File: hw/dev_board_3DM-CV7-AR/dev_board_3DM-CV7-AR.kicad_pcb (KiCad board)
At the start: 4 copper layers, 26 parts, among them J1 87438-0643, U1 DMP2240UW, U2 DMP2240UW

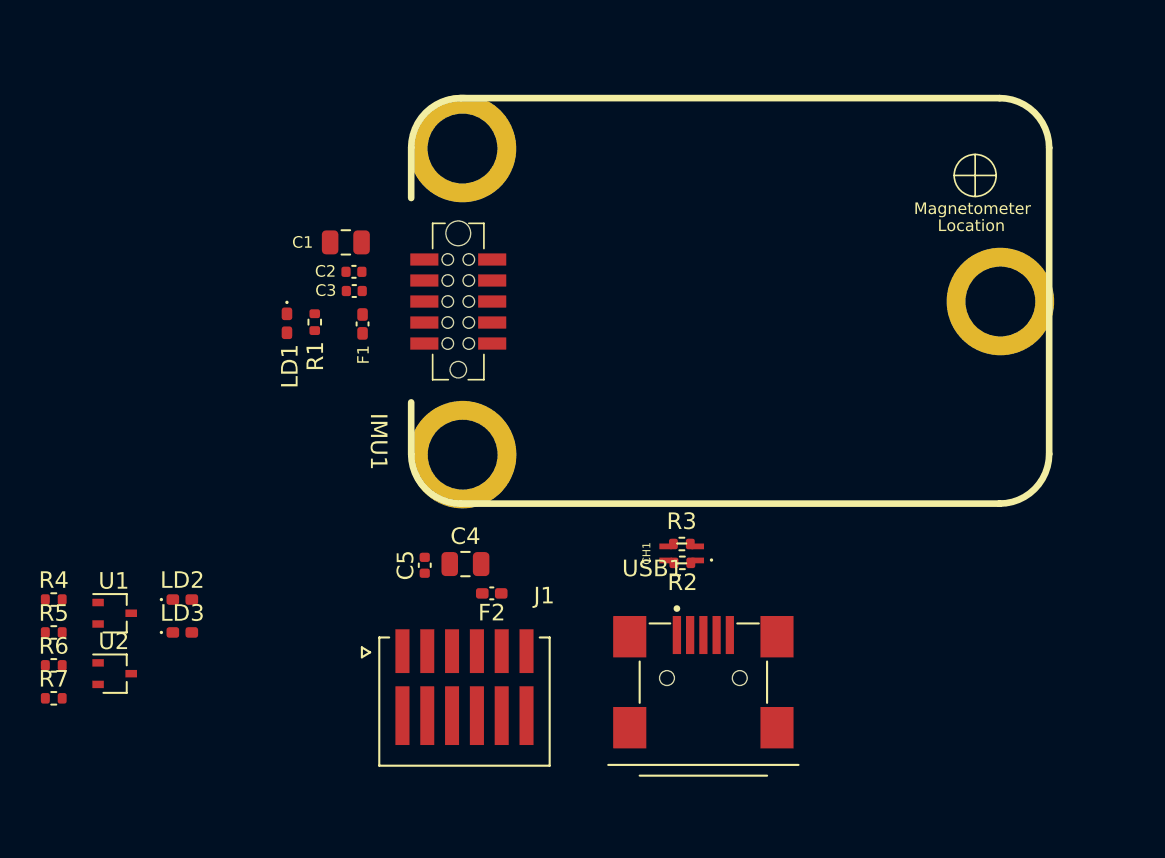
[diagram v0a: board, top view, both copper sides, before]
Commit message: Finalizado
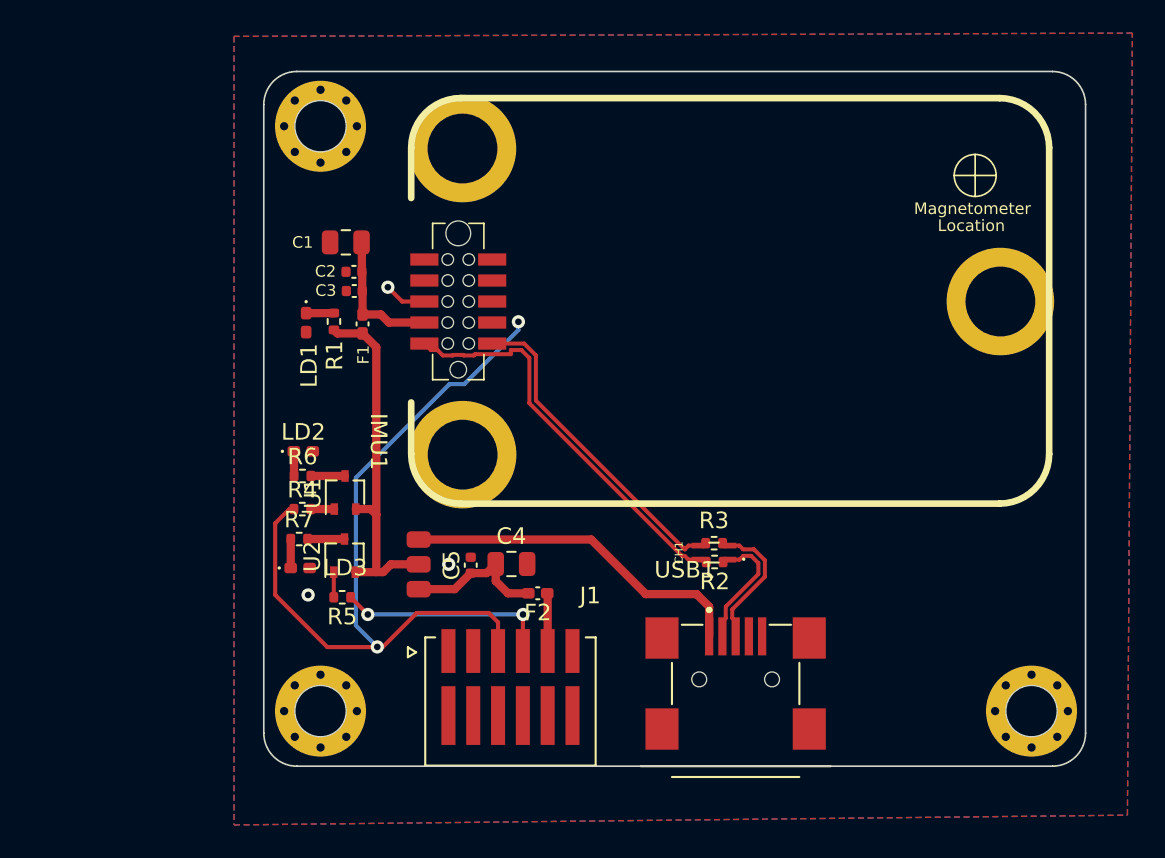
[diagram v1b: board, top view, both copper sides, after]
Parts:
- added MC4: M3_Hole, Herranz - Various:M3_Hole, F.Cu at (157.4, 122.0)
- added MC5: M3_Hole, Herranz - Various:M3_Hole, F.Cu at (114.4, 86.7)
- added MC6: M3_Hole, Herranz - Various:M3_Hole, F.Cu at (114.4, 122.0)
- added SEL1: ~, Herranz - Various:pad_selector, F.Cu at (120.3, 113.2)
- moved R6 18.9 mm to (113.3, 107.8)
- moved R7 17.7 mm to (113.1, 111.7)
- moved R5 17.6 mm to (115.7, 115.2), turned to 180 degrees
- moved R4 16.0 mm to (113.3, 109.8)
- moved U1 15.7 mm to (115.9, 108.8), turned to 90 degrees
- moved U2 15.6 mm to (115.9, 112.7), turned to 90 degrees
- moved LD2 11.6 mm to (113.4, 106.3)
- moved LD3 8.12 mm to (113.2, 113.4)
- moved C4 2.78 mm to (125.9, 113.2)
- moved C5 2.78 mm to (123.5, 113.2)
- moved F2 2.78 mm to (127.5, 114.9)
- moved J1 2.78 mm to (125.9, 113.2)
- moved USB1 1.95 mm to (139.5, 117.6)
- moved CH1 1.95 mm to (138.2, 112.5)
- moved R2 1.95 mm to (138.2, 113.0)
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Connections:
- net Net-(USB1-D+) renamed /D_conn+
- net Net-(USB1-D-) renamed /D_conn-
- F1 pad 1: +3V3 -> +5VD
- MC3 pad 1: GND -> unconnected-(MC3-Pad1)
- R1 pad 2: +3V3 -> +5VD
- R6 pad 2: Net-(U1-S) -> Net-(U1-D)
- R7 pad 2: Net-(U2-S) -> Net-(U2-D)
- U1 pad 2: Net-(U1-S) -> +5VD
- U1 pad 3: +3V3 -> Net-(U1-D)
- U2 pad 2: Net-(U2-S) -> +5VD
- U2 pad 3: +3V3 -> Net-(U2-D)
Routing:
- net /Rx: track 0.00 -> 48.2 mm, vias 0 -> 2
- net /Tx: track 0.00 -> 35.9 mm, vias 0 -> 3
- net /D-: track 0.00 -> 24.0 mm
- net +5VD: track 0.00 -> 22.0 mm
- net VBUS: track 0.00 -> 21.0 mm
- net /D+: track 0.00 -> 19.3 mm
- net +5V: track 0.00 -> 8.59 mm
- net Net-(IMU1-VCC): track 0.00 -> 8.32 mm
- net /D_conn+: track 0.00 -> 7.97 mm
- net /D_conn-: track 0.00 -> 7.31 mm
- net Net-(J1-Pin_5): track 0.00 -> 3.50 mm
- net Net-(U2-D): track 0.00 -> 2.23 mm
- net Net-(U1-D): track 0.00 -> 2.06 mm
- net Net-(LD3-A): track 0.00 -> 1.75 mm
- net Net-(LD1-A): track 0.00 -> 1.68 mm
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- added copper zone on B.Cu, net GND
- added copper zone on F.Cu, net GND
- added copper zone on In1.Cu, net GND
- added copper zone on In2.Cu, net GND
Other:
- board outline added: 49.7 x 42 mm
